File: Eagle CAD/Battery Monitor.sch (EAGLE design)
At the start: 7 parts

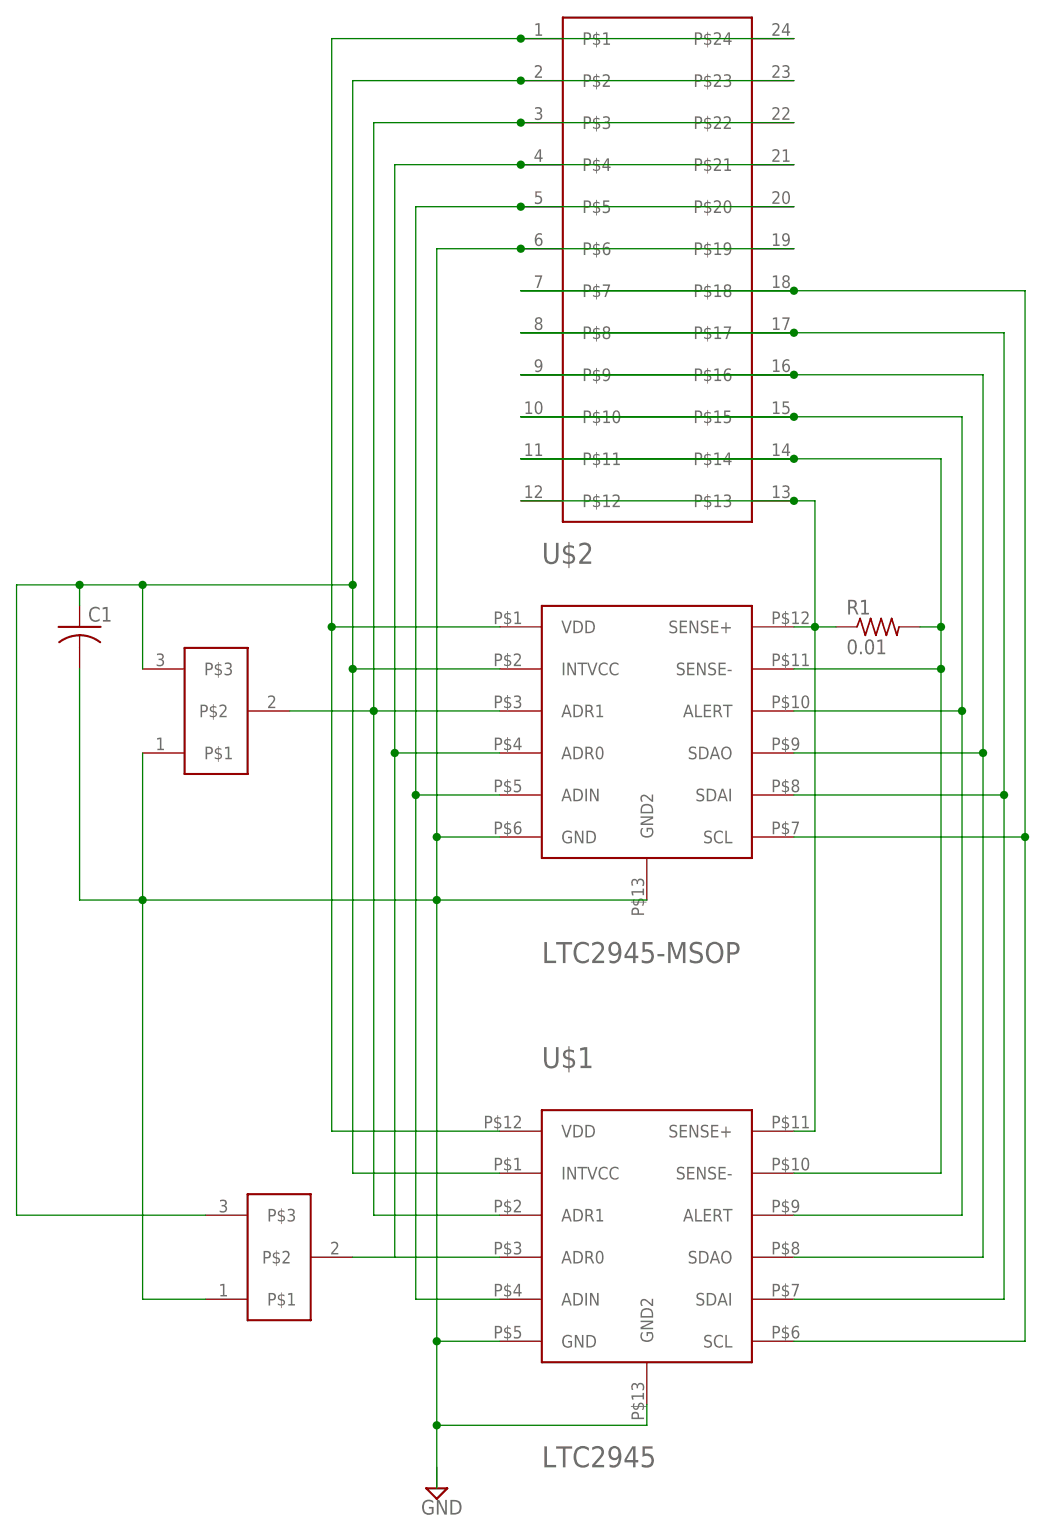
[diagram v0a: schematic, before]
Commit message: Finalized.
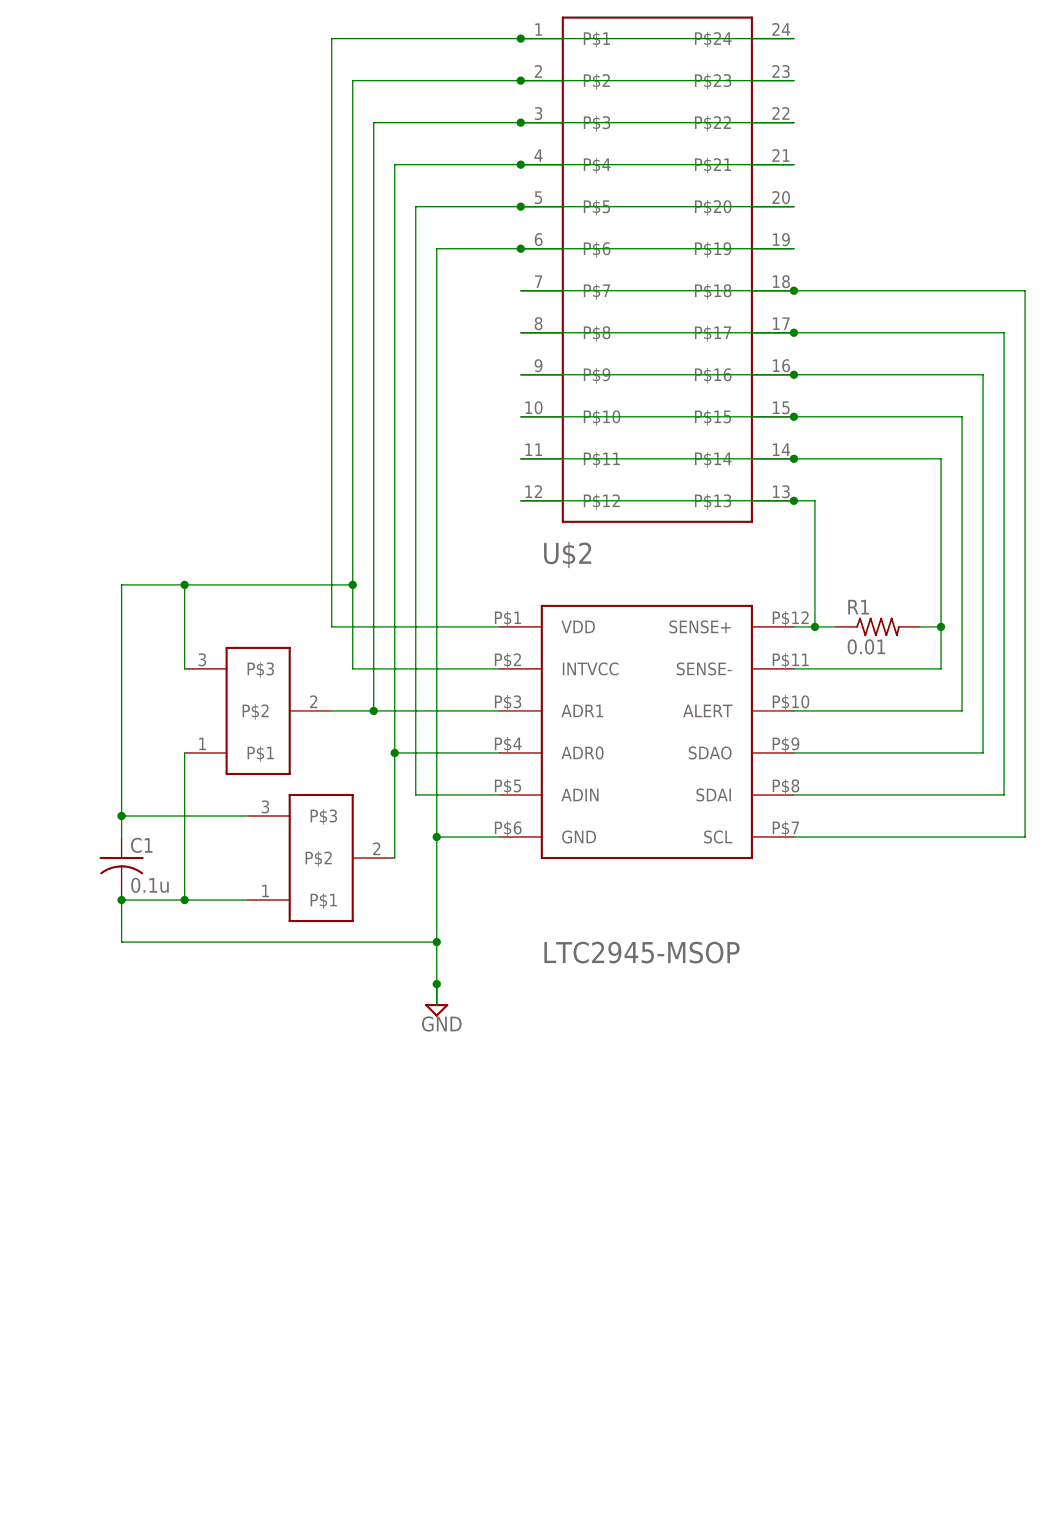
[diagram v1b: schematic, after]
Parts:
- removed U$1: LTC2945, Raj:LTC2945
- C1: value (none) -> 0.1u
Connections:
- removed net N$1: C1.2, U$1.GND, U$1.GND2, U$2.GND, U$2.GND2, U$3.P$19, U$3.P$6, U$4.P$1, U$5.P$1
- new net GND: C1.2, U$2.GND, U$3.P$19, U$3.P$6, U$4.P$1, U$5.P$1
- net N$10: no longer U$1.ALERT
- net N$11: no longer U$1.SENSE-
- net N$14: no longer U$1.SDAI
- net N$2: no longer U$1.INTVCC
- net N$3: no longer U$1.VDD
- net N$4: no longer U$1.ADR1
- net N$5: no longer U$1.ADR0
- net N$6: no longer U$1.ADIN
- net N$7: no longer U$1.SCL
- net N$8: no longer U$1.SDAO
- net N$9: no longer U$1.SENSE+
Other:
- moved on the sheet: C1
